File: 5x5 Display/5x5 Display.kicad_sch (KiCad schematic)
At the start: 58 parts, among them U3 DRV1

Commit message: buck layout
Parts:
- NT1, NT2: footprint NetTie:NetTie-2_THT_Pad1.0mm -> NetTie:NetTie-2_SMD_Pad0.5mm
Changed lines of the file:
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@@
 			)
 		)
-		(property "Footprint" "NetTie:NetTie-2_THT_Pad1.0mm"
+		(property "Footprint" "NetTie:NetTie-2_SMD_Pad0.5mm"
 			(at 196.85 45.72 0)
 			(effects
@@
 			)
 		)
-		(property "Footprint" "NetTie:NetTie-2_THT_Pad1.0mm"
+		(property "Footprint" "NetTie:NetTie-2_SMD_Pad0.5mm"
 			(at 196.85 90.17 0)
 			(effects

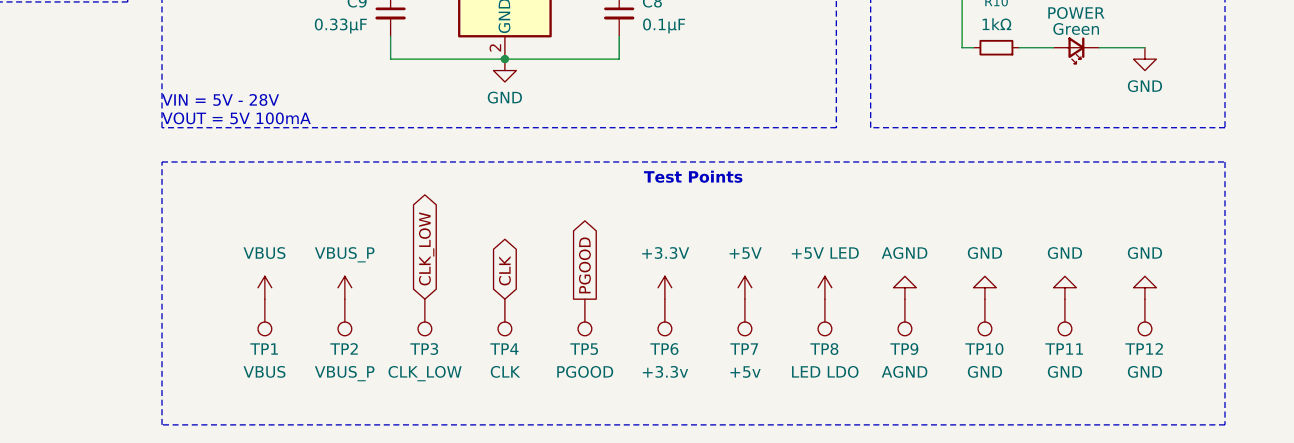
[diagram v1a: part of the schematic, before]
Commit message: Initial route complete
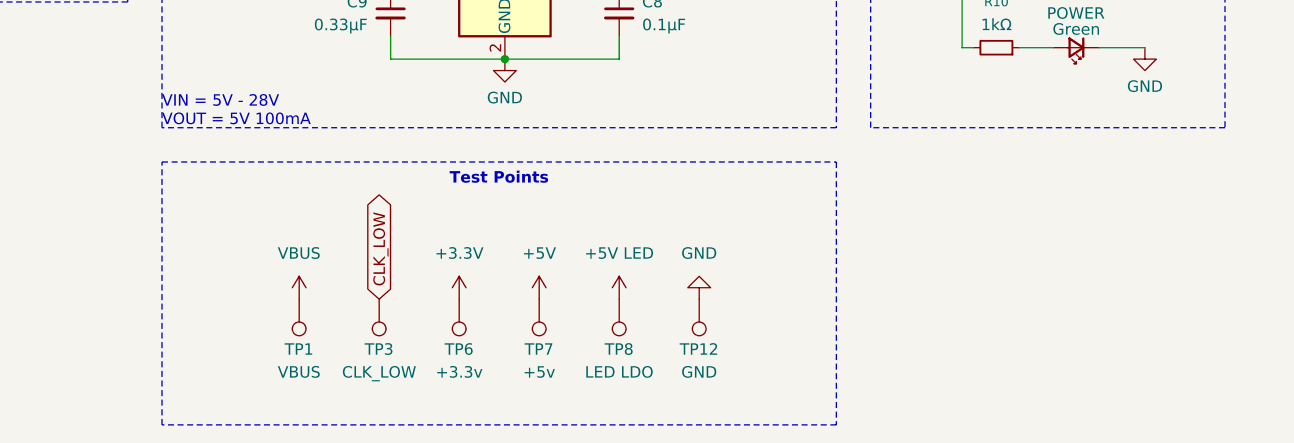
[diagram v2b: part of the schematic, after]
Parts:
- removed TP10, TP11: GND, TestPoint:TestPoint_Pad_D1.5mm, symbol Connector:TestPoint
- removed TP2: VBUS_P, TestPoint:TestPoint_Pad_D1.5mm, symbol Connector:TestPoint
- removed TP4: CLK, TestPoint:TestPoint_Pad_D1.5mm, symbol Connector:TestPoint
- removed TP5: PGOOD, TestPoint:TestPoint_Pad_D1.5mm, symbol Connector:TestPoint
- removed TP9: AGND, TestPoint:TestPoint_Pad_D1.5mm, symbol Connector:TestPoint
- D10: now left out of the parts list
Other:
- moved on the sheet: TP1, TP12, TP3, TP6, TP7, TP8
